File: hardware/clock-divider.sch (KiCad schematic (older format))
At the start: 16 parts, among them J1 PWR, J2 Serial debug / programming he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, J3 SPI / ICSP header, U1 ATmega328P-PU, Y1 16MHz

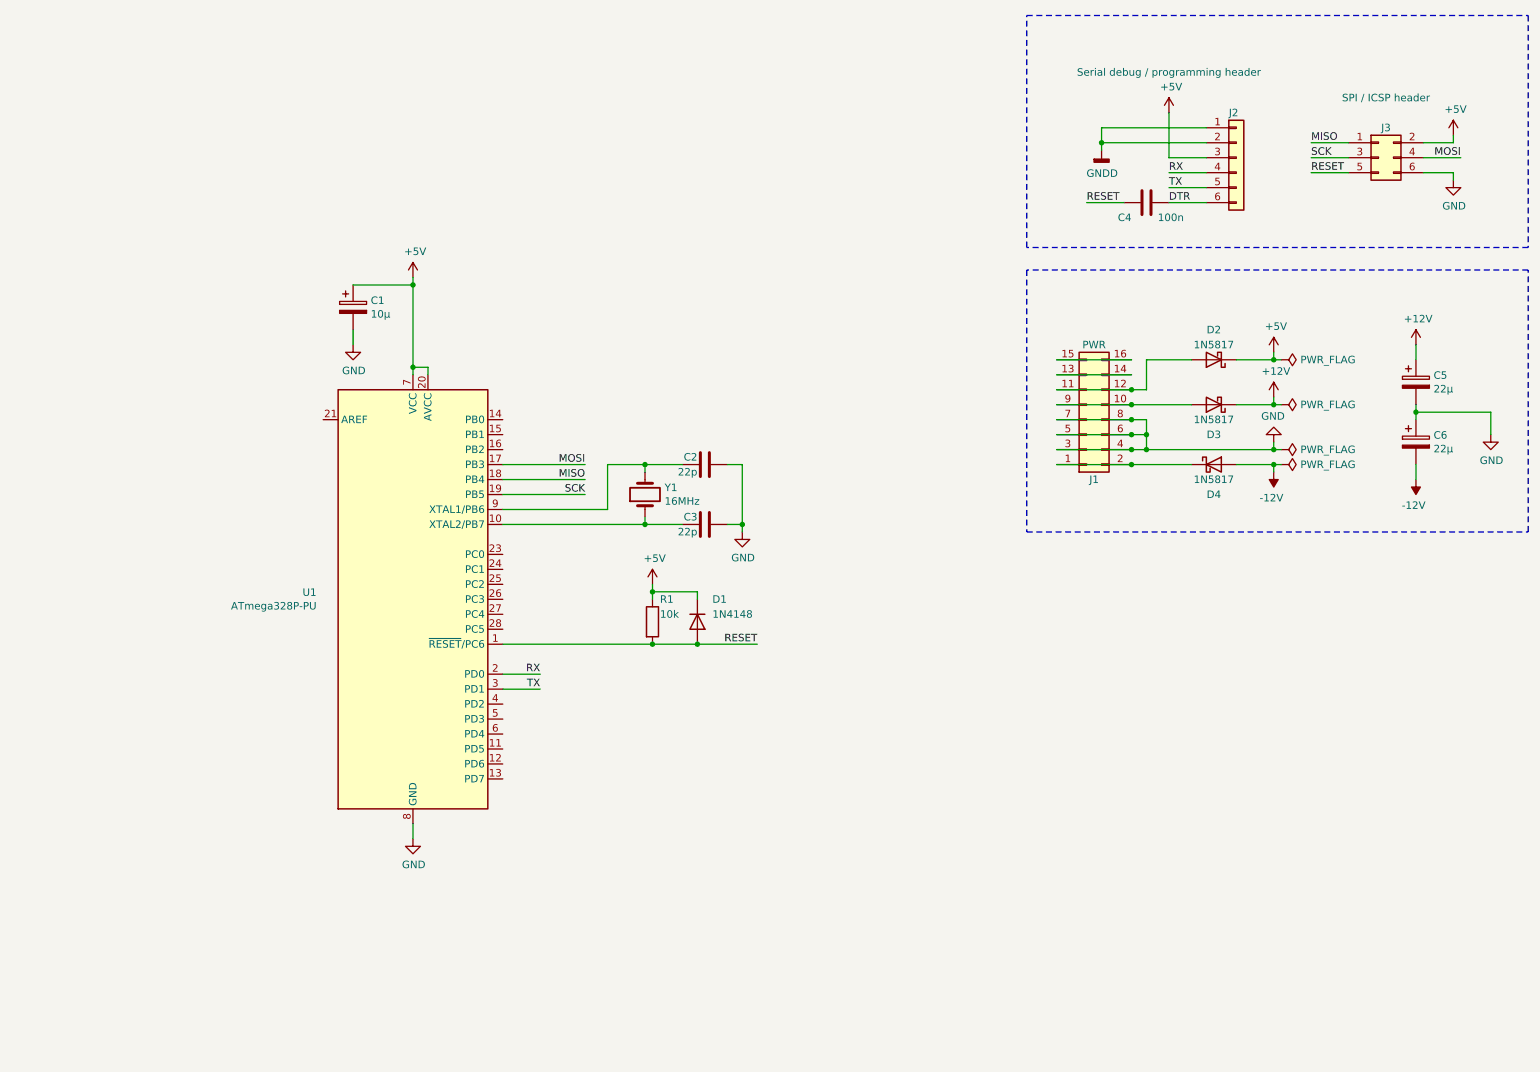
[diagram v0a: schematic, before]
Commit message: continue schematic
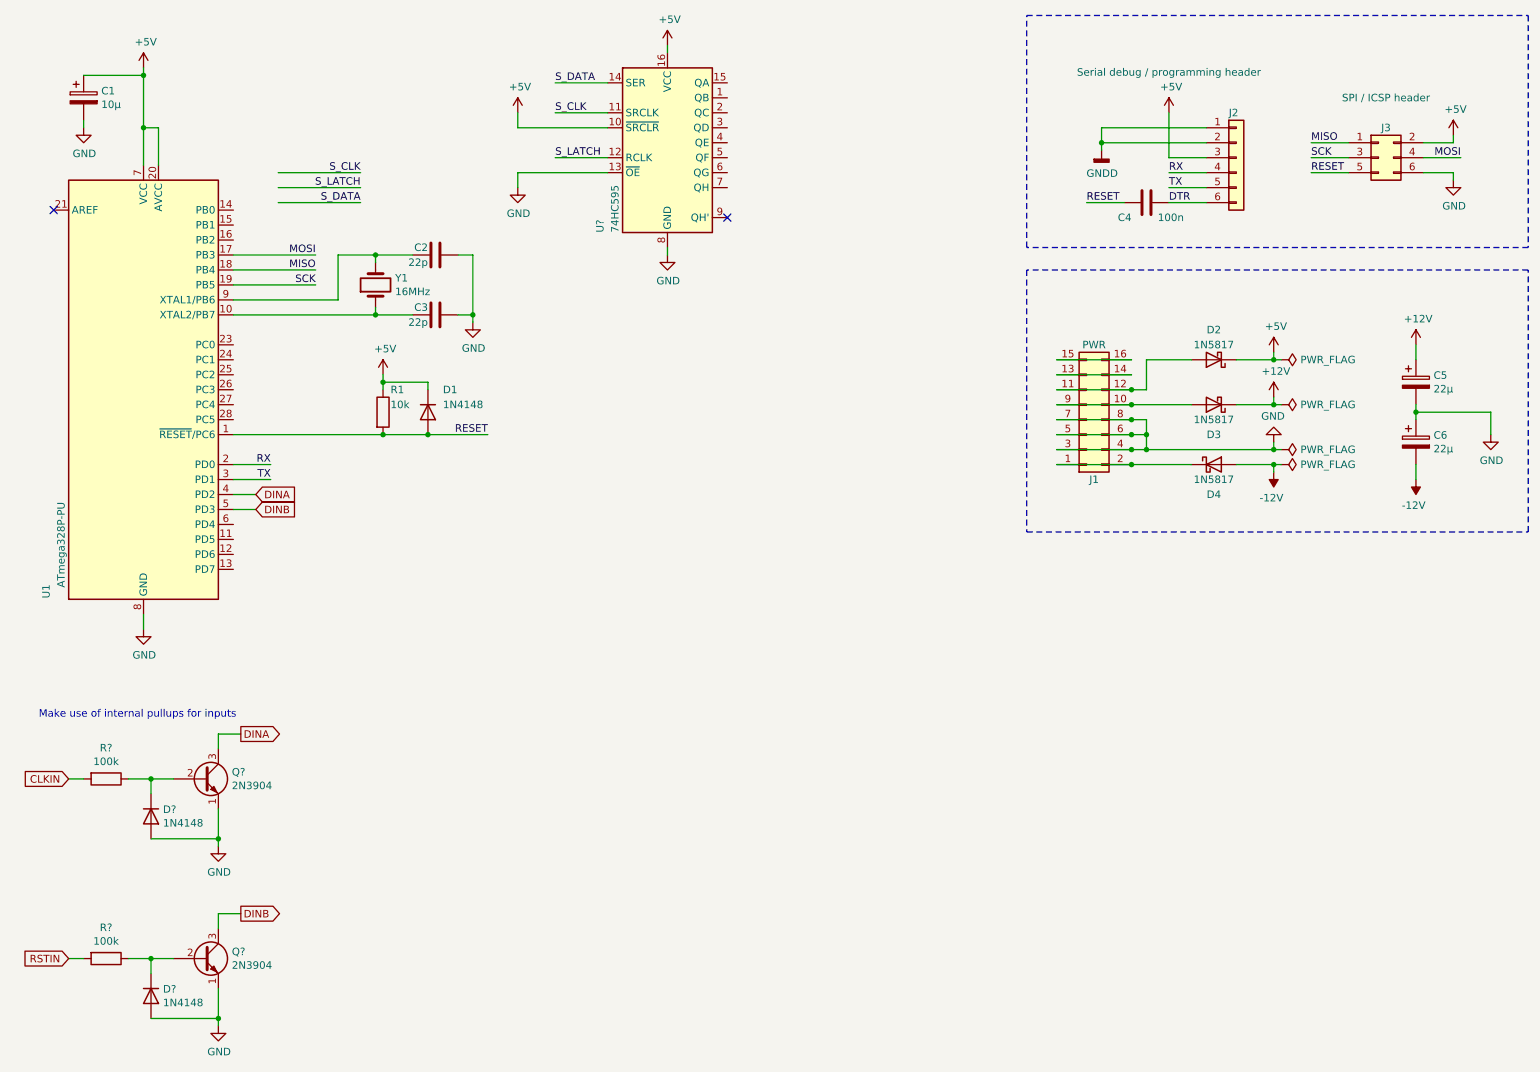
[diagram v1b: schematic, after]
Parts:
- added D? (x2): 1N4148, Diode_THT:D_DO-35_SOD27_P7.62mm_Horizontal, symbol Diode:1N4148
- added Q? (x2): 2N3904, Package_TO_SOT_THT:TO-92_Inline, symbol Transistor_BJT:2N3904
- added R? (x2): 100k, symbol Device:R
- added U?: 74HC595, symbol 74xx:74HC595
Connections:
- net +5V: now also U?.10 (~SRCLR), U?.16 (VCC)
- net GND: now also D?.2 (A), D?.2 (A), Q?.1 (E), Q?.1 (E), U?.13 (~OE), U?.8 (GND)
- net DINA: now reaches U1.4 (PD2)
- net DINA: now also Q?.3 (C)
- net DINB: now reaches U1.5 (PD3)
- net DINB: now also Q?.3 (C)
- new net: D?.1 (K), Q?.2 (B), R?.1 (x2)
- new net CLKIN: R?.2
- new net RSTIN: R?.2
- new net S_CLK: U?.11 (SRCLK)
- new net S_DATA: U?.14 (SER)
- new net S_LATCH: U?.12 (RCLK)
- no-connect marks 0 -> 2
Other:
- note added: "Make use of internal pullups for inputs"
- moved on the sheet: C1, C2, C3, D1, R1, U1, Y1
